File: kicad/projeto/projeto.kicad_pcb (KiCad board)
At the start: 2 copper layers, 123.2 x 127 mm, 57 parts, among them Q1 BTA16-600B, Q2 BTA16-600B, U1 ESP-12E, U3v3 LM1117-3.3

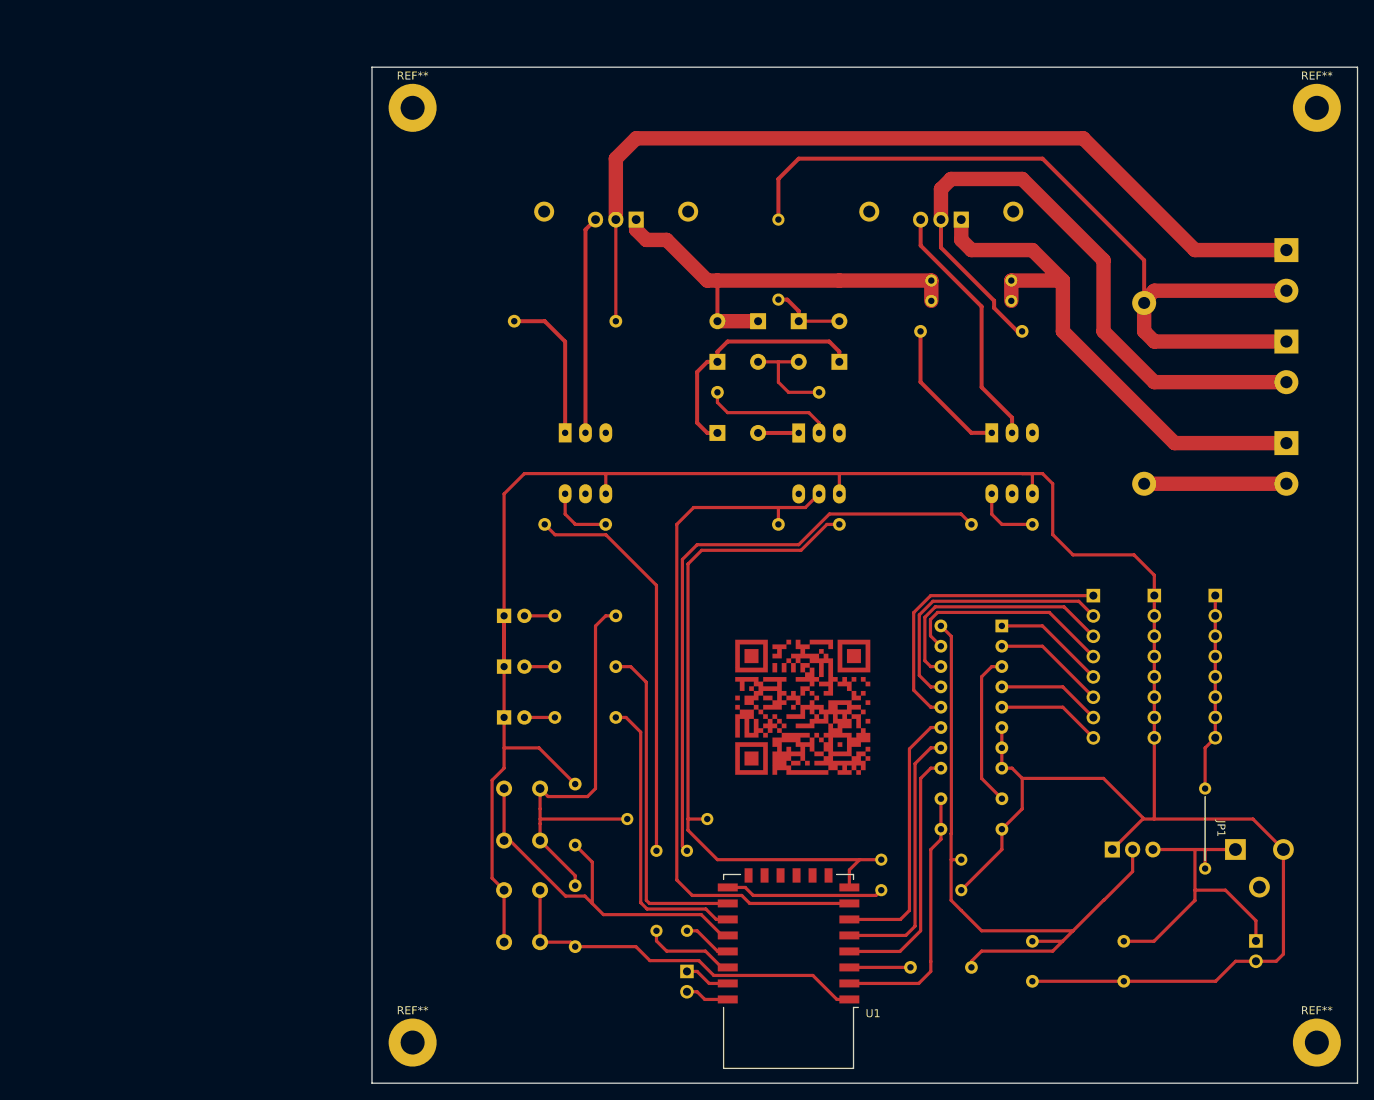
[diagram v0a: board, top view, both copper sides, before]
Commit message: Add alguns dados na pcb
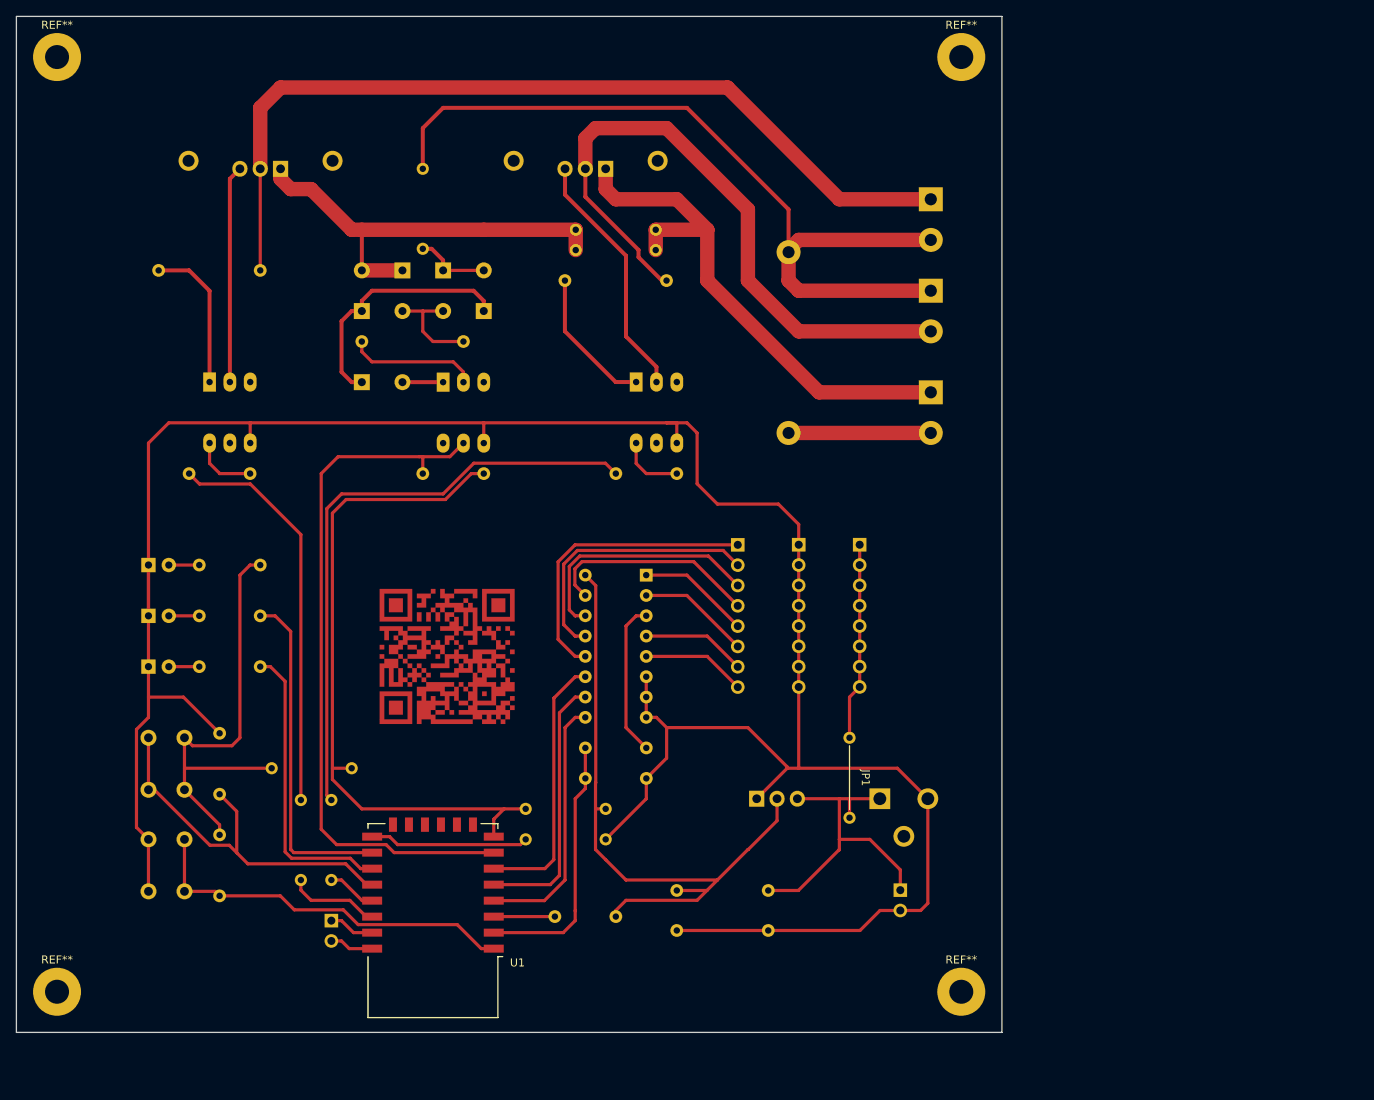
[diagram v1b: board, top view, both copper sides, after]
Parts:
- moved D2 44.9 mm to (137.2, 59.7)
- moved JP5 44.9 mm to (157.5, 127.0)
- moved JP6 44.9 mm to (147.5, 130.8)
- moved JP8 44.9 mm to (119.4, 125.9)
- moved Jpwr_sens1 44.9 mm to (189.2, 94.0)
- moved Q1 44.9 mm to (157.5, 47.0)
- moved Ren1 44.9 mm to (151.1, 140.5)
- moved Rtriac1 44.9 mm to (152.4, 61.0)
- moved Rtriac2 44.9 mm to (101.6, 59.7)
- moved U1 44.9 mm to (135.9, 141.0)
- moved Udet_0 44.9 mm to (137.2, 73.7)
- moved Uload1 44.9 mm to (161.3, 73.6)
- moved Don1 44.9 mm to (100.3, 96.5)
- moved Dss1 44.9 mm to (100.3, 102.9)
- moved Dwifi1 44.9 mm to (100.3, 109.2)
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
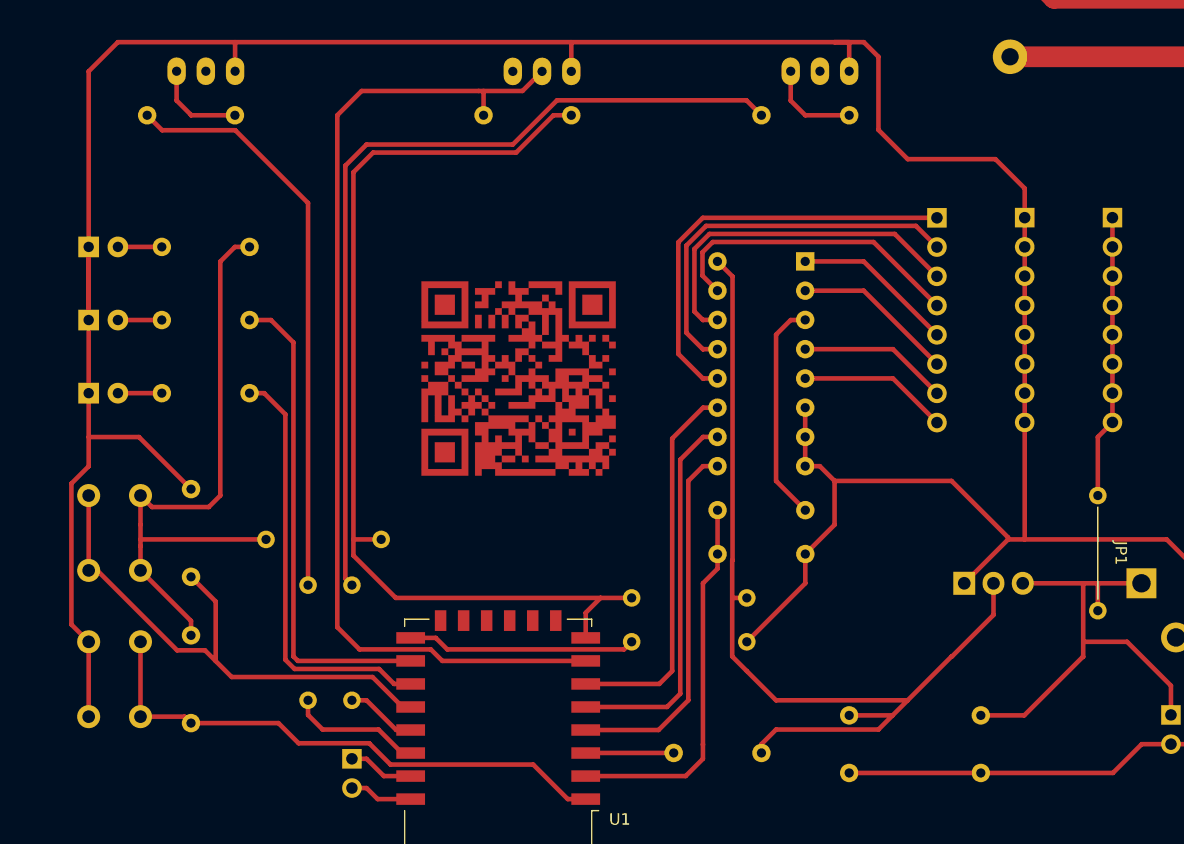
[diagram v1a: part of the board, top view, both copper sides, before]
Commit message: Fix PCB
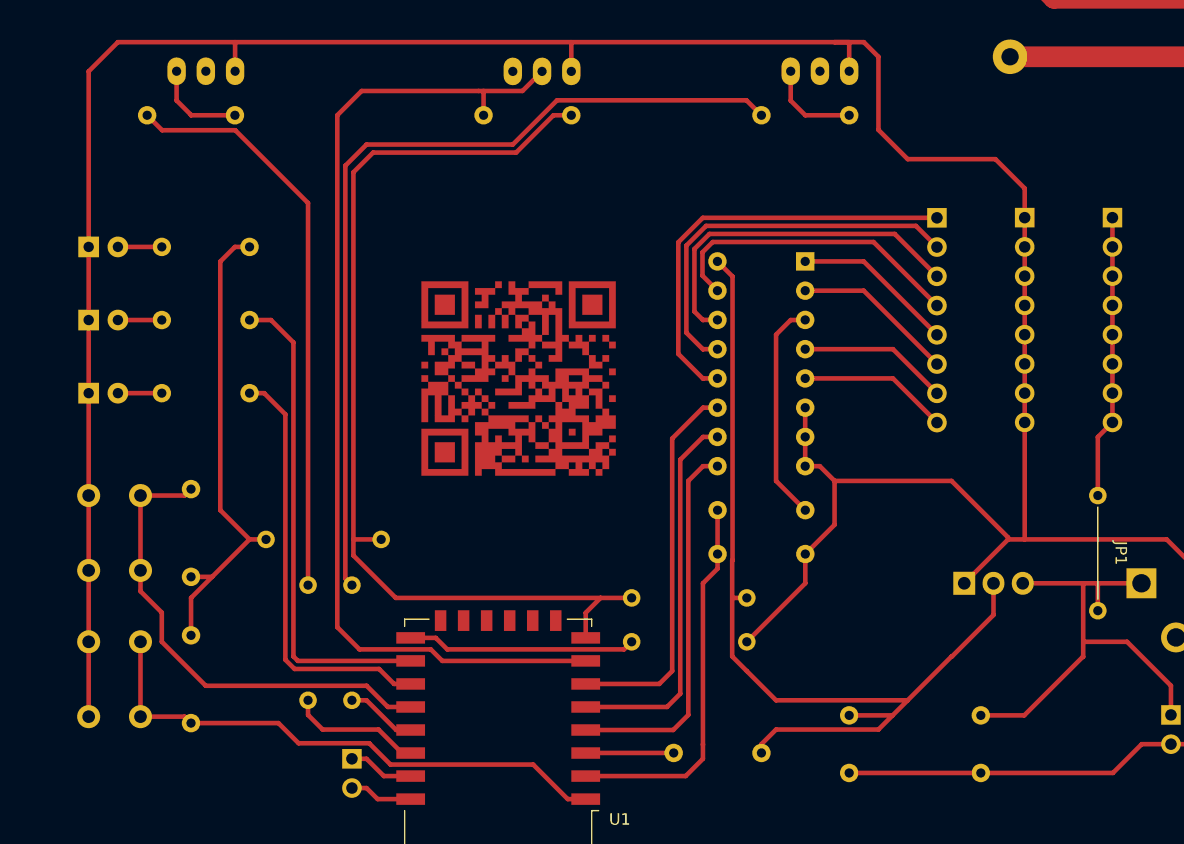
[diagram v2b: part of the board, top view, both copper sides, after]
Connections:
- Rexit1 pad 1: /exit_intr -> /3v3'2
- Rexit1 pad 2: GND -> /exit_intr
- SWexit1 pad 1: /3v3'2 -> /exit_intr
- SWexit1 pad 2: /exit_intr -> GND
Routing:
- net GND: track 317.3 -> 299.7 mm
- net /3v3'2: track 56.0 -> 41.9 mm
- net /exit_intr: track 47.6 -> 42.0 mm
- net /multiplex_C: track 32.1 -> 32.8 mm
